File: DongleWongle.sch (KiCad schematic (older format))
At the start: 28 parts

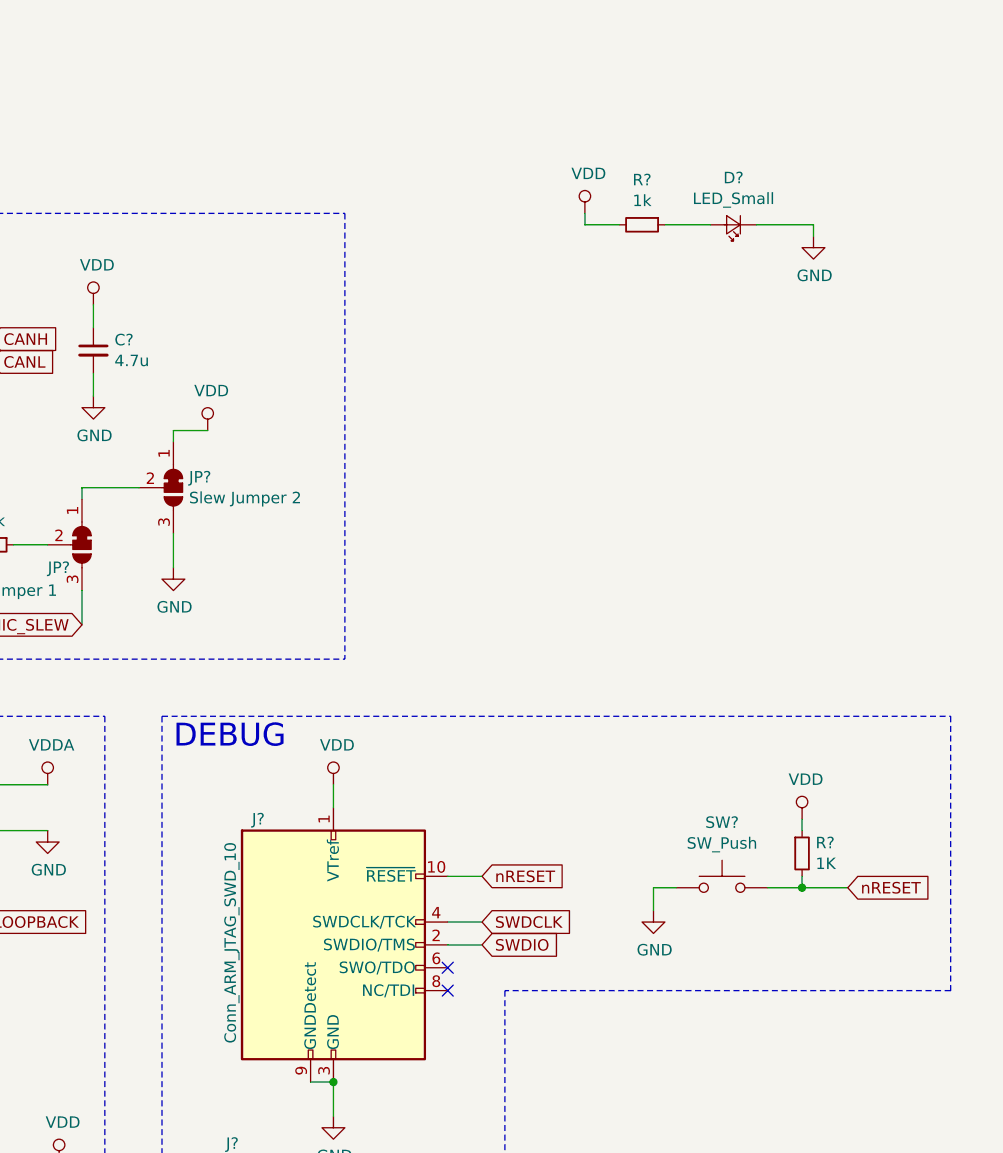
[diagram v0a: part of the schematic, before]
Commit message: add power
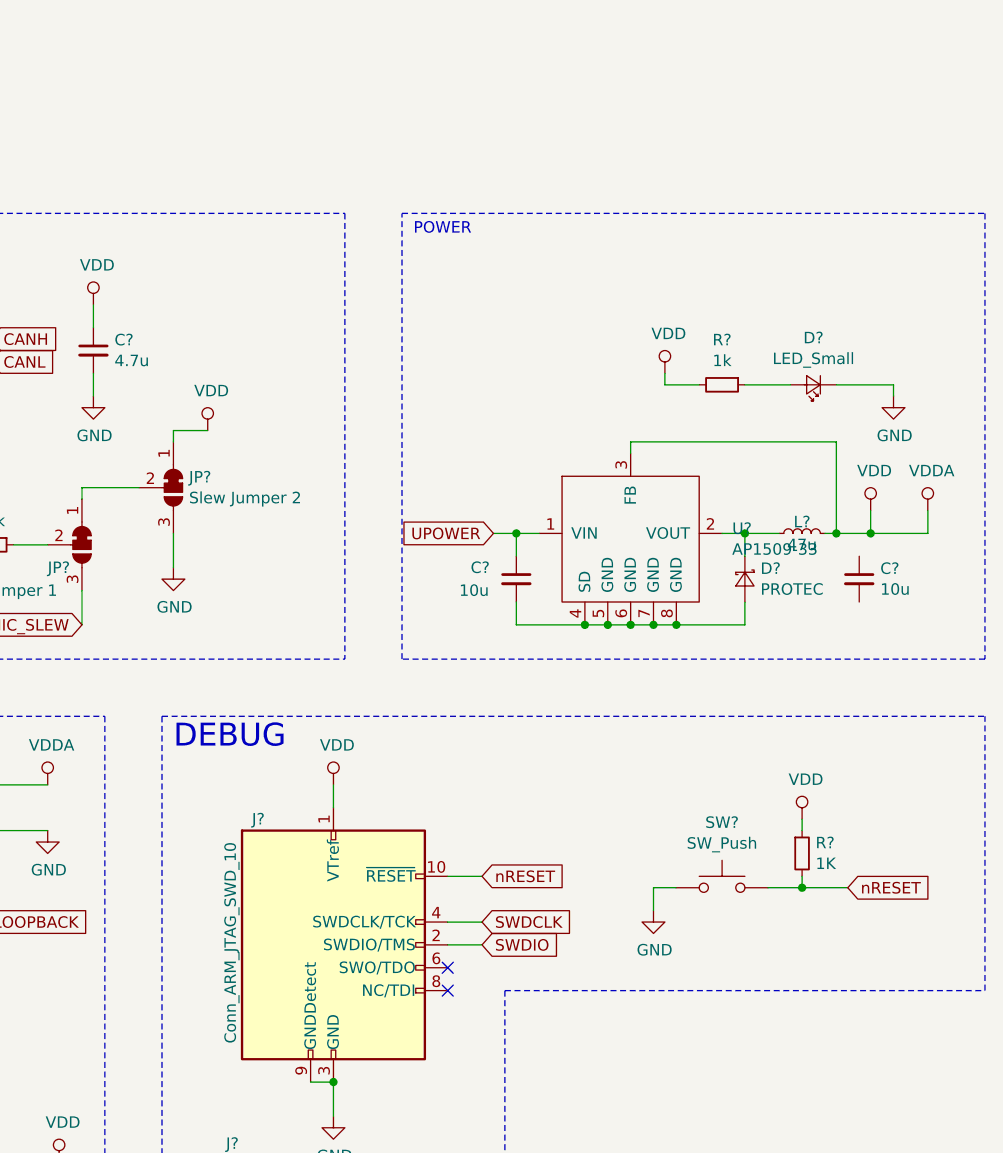
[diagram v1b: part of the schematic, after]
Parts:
- added C? (x2): 10u, symbol Device:C_Small
- added D?: PROTEC, symbol Device:D_Schottky_Small
- added L?: 47u, symbol Device:L_Small
- added U?: AP1509-33, symbol star-sch-block-symbols:AP1509-33
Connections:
- net VDDA is gone; now on net VDD: C?.1, C?.1, U?.5 (VDDA)
- net UPOWER: now also C?.1, U?.1 (VIN)
- net VDD: now also L?.2, U?.3 (FB)
- new net: D?.1 (K), L?.1, U?.2 (VOUT)
- new net: C?.2, D?.2 (A), U?.4 (SD), U?.5 (GND), U?.6 (GND), U?.7 (GND), U?.8 (GND)
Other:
- note added: "POWER"
- moved on the sheet: D?, R?
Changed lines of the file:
@@
 L power:GND #PWR?
 U 1 1 5EB5DE63
-P 8100 3050
-F 0 "#PWR?" H 8100 2800 50  0001 C CNN
-F 1 "GND" H 8105 2877 50  0000 C CNN
-F 2 "" H 8100 3050 50  0001 C CNN
-F 3 "" H 8100 3050 50  0001 C CNN
-	1    8100 3050
+P 8450 3750
+F 0 "#PWR?" H 8450 3500 50  0001 C CNN
+F 1 "GND" H 8455 3577 50  0000 C CNN
+F 2 "" H 8450 3750 50  0001 C CNN
+F 3 "" H 8450 3750 50  0001 C CNN
+	1    8450 3750
 	1    0    0    -1
 $EndComp
@@
 L power:VDD #PWR?
 U 1 1 5EB5E1C3
-P 7100 2950
-F 0 "#PWR?" H 7100 2800 50  0001 C CNN
-F 1 "VDD" H 7117 3123 50  0000 C CNN
-F 2 "" H 7100 2950 50  0001 C CNN
-F 3 "" H 7100 2950 50  0001 C CNN
-	1    7100 2950
+P 7450 3650
+F 0 "#PWR?" H 7450 3500 50  0001 C CNN
+F 1 "VDD" H 7467 3823 50  0000 C CNN
+F 2 "" H 7450 3650 50  0001 C CNN
+F 3 "" H 7450 3650 50  0001 C CNN
+	1    7450 3650
 	1    0    0    -1
 $EndComp
@@
 L Device:R_Small R?
 U 1 1 5EB6A610
-P 7350 3000
-F 0 "R?" V 7154 3000 50  0000 C CNN
-F 1 "1k" V 7245 3000 50  0000 C CNN
-F 2 "" H 7350 3000 50  0001 C CNN
-F 3 "~" H 7350 3000 50  0001 C CNN
-	1    7350 3000
+P 7700 3700
+F 0 "R?" V 7504 3700 50  0000 C CNN
+F 1 "1k" V 7595 3700 50  0000 C CNN
+F 2 "" H 7700 3700 50  0001 C CNN
+F 3 "~" H 7700 3700 50  0001 C CNN
+	1    7700 3700
 	0    1    1    0
 $EndComp
@@
 L Device:LED_Small D?
 U 1 1 5EB6C3D4
-P 7750 3000
-F 0 "D?" H 7750 2795 50  0000 C CNN
-F 1 "LED_Small" H 7750 2886 50  0000 C CNN
-F 2 "" V 7750 3000 50  0001 C CNN
-F 3 "~" V 7750 3000 50  0001 C CNN
-	1    7750 3000
+P 8100 3700
+F 0 "D?" H 8100 3495 50  0000 C CNN
+F 1 "LED_Small" H 8100 3586 50  0000 C CNN
+F 2 "" V 8100 3700 50  0001 C CNN
+F 3 "~" V 8100 3700 50  0001 C CNN
+	1    8100 3700
 	-1   0    0    1
 $EndComp
 Wire Wire Line
-	8100 3050 8100 3000
-Wire Wire Line
-	8100 3000 7850 3000
-Wire Wire Line
-	7650 3000 7450 3000
-Wire Wire Line
-	7100 2950 7100 3000
-Wire Wire Line
-	7100 3000 7250 3000
+	8450 3750 8450 3700
+Wire Wire Line
+	8450 3700 8200 3700
+Wire Wire Line
+	8000 3700 7800 3700
+Wire Wire Line
+	7450 3650 7450 3700
+Wire Wire Line
+	7450 3700 7600 3700
 $Comp
 L Connector:TestPoint TP?
@@
 Wire Notes Line
 	6050 2950 6050 4900
-Wire Notes Line
-	5250 5150 8700 5150
 Text Notes 5300 5300 0    100  ~ 0
 DEBUG
@@
 	750  5150 750  7600
 Wire Notes Line
-	8700 5150 8700 6350
-Wire Notes Line
-	8700 6350 6750 6350
-Wire Notes Line
 	6750 6350 6750 7600
 Wire Notes Line
@@
 Wire Notes Line
 	5250 5150 5250 7600
+$Comp
+L power:VDD #PWR?
+U 1 1 5EF519DD
+P 8350 4250
+F 0 "#PWR?" H 8350 4100 50  0001 C CNN
+F 1 "VDD" H 8367 4423 50  0000 C CNN
+F 2 "" H 8350 4250 50  0001 C CNN
+F 3 "" H 8350 4250 50  0001 C CNN
+	1    8350 4250
+	1    0    0    -1
+$EndComp
+$Comp
+L power:VDDA #PWR?
+U 1 1 5EF53BED
+P 8600 4250
+F 0 "#PWR?" H 8600 4100 50  0001 C CNN
+F 1 "VDDA" H 8617 4423 50  0000 C CNN
+F 2 "" H 8600 4250 50  0001 C CNN
+F 3 "" H 8600 4250 50  0001 C CNN
+	1    8600 4250
+	1    0    0    -1
+$EndComp
+Wire Wire Line
+	8600 4350 8350 4350
+Wire Wire Line
+	8600 4250 8600 4350
+Wire Wire Line
+	8350 4350 8350 4250
+$Comp
+L Device:L_Small L?
+U 1 1 5EF77160
+P 8050 4350
+F 0 "L?" V 8100 4350 50  0000 C CNN
+F 1 "47u" V 8000 4350 50  0000 C CNN
+F 2 "" H 8050 4350 50  0001 C CNN
+F 3 "~" H 8050 4350 50  0001 C CNN
+	1    8050 4350
+	0    -1   -1   0
+$EndComp
+Wire Wire Line
+	7950 4350 7800 4350
+Wire Wire Line
+	8150 4350 8200 4350
+Connection ~ 8350 4350
+$Comp
+L Device:D_Schottky_Small D?
+U 1 1 5EF87033
+P 7800 4550
+F 0 "D?" V 7754 4618 50  0000 L CNN
+F 1 "PROTEC" V 7845 4618 50  0000 L CNN
+F 2 "" V 7800 4550 50  0001 C CNN
+F 3 "~" V 7800 4550 50  0001 C CNN
+	1    7800 4550
+	0    1    1    0
+$EndComp
+Wire Wire Line
+	7800 4350 7800 4450
+Connection ~ 7800 4350
+Wire Wire Line
+	7800 4350 7700 4350
+Wire Wire Line
+	7800 4650 7800 4750
+Wire Wire Line
+	8200 4350 8200 3950
+Wire Wire Line
+	8200 3950 7300 3950
+Wire Wire Line
+	7300 3950 7300 4000
+Connection ~ 8200 4350
+Wire Wire Line
+	8200 4350 8350 4350
+$Comp
+L Device:C_Small C?
+U 1 1 5EFBA513
+P 8300 4550
+F 0 "C?" H 8392 4596 50  0000 L CNN
+F 1 "10u" H 8392 4505 50  0000 L CNN
+F 2 "" H 8300 4550 50  0001 C CNN
+F 3 "~" H 8300 4550 50  0001 C CNN
+	1    8300 4550
+	1    0    0    -1
+$EndComp
+$Comp
+L Device:C_Small C?
+U 1 1 5EFBB885
+P 6800 4550
+F 0 "C?" H 6600 4600 50  0000 L CNN
+F 1 "10u" H 6550 4500 50  0000 L CNN
+F 2 "" H 6800 4550 50  0001 C CNN
+F 3 "~" H 6800 4550 50  0001 C CNN
+	1    6800 4550
+	1    0    0    -1
+$EndComp
+Wire Wire Line
+	6800 4650 6800 4750
+Wire Wire Line
+	6900 4350 6800 4350
+Wire Wire Line
+	6800 4350 6800 4450
+Text GLabel 6700 4350 0    50   Input ~ 0
+UPOWER
+Wire Wire Line
+	6700 4350 6800 4350
+Connection ~ 6800 4350
+Wire Notes Line
+	6300 4900 6300 2950
+Wire Notes Line
+	8850 2950 8850 4900
+Wire Notes Line
+	8850 4900 6300 4900
+Wire Notes Line
+	6300 2950 8850 2950
+Wire Notes Line
+	8850 6350 8850 5150
+Wire Notes Line
+	5250 5150 8850 5150
+Wire Notes Line
+	6750 6350 8850 6350
+Text Notes 6350 3050 0    50   ~ 0
+POWER
+Wire Wire Line
+	6800 4750 7100 4750
+$Comp
+L star-sch-block-symbols:AP1509-33 U?
+U 1 1 5F0A0CB9
+P 7300 4300
+F 0 "U?" H 7744 4271 50  0000 L CNN
+F 1 "AP1509-33" H 7744 4180 50  0000 L CNN
+F 2 "" H 7350 4650 50  0001 C CNN
+F 3 "https://www.diodes.com/assets/Datasheets/AP1509.pdf" H 7350 4650 50  0001 C CNN
+	1    7300 4300
+	1    0    0    -1
+$EndComp
+Wire Wire Line
+	7500 4750 7800 4750
+Wire Wire Line
+	7500 4750 7400 4750
+Connection ~ 7500 4750
+Wire Wire Line
+	7400 4750 7300 4750
+Connection ~ 7400 4750
+Wire Wire Line
+	7100 4750 7200 4750
+Connection ~ 7100 4750
+Connection ~ 7200 4750
+Wire Wire Line
+	7200 4750 7300 4750
+Connection ~ 7300 4750
 $EndSCHEMATC
